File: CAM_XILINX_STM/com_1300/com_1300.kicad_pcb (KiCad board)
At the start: 6 copper layers, 50 x 75.9 mm, 113 parts, among them IC1 XC3S400-4TQ144C, J1 MEC1-108-01-S-D-RA1-SL, J2 Conn_02x10_Top_Bottom, J3 9-68RD-0.635SF, U1 LT1963AxST-3.3, U2 LP3982IMM-ADJ, U3 LTC3411EMS, U4 STM32F415RGTx, U5 AM29LV320DT90EC, U6 TC74LCX373FT, Y1 40mHZ, Y2 16mHz

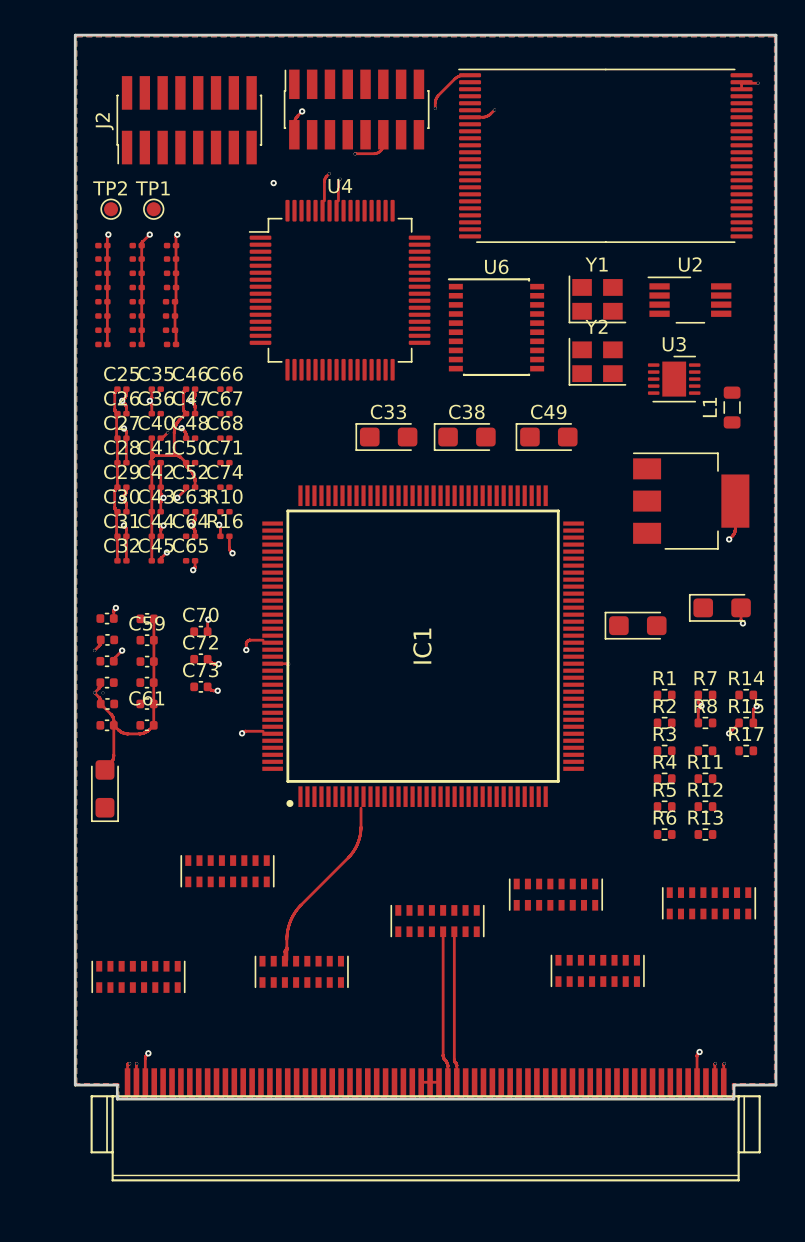
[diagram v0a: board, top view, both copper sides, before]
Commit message: 23623637
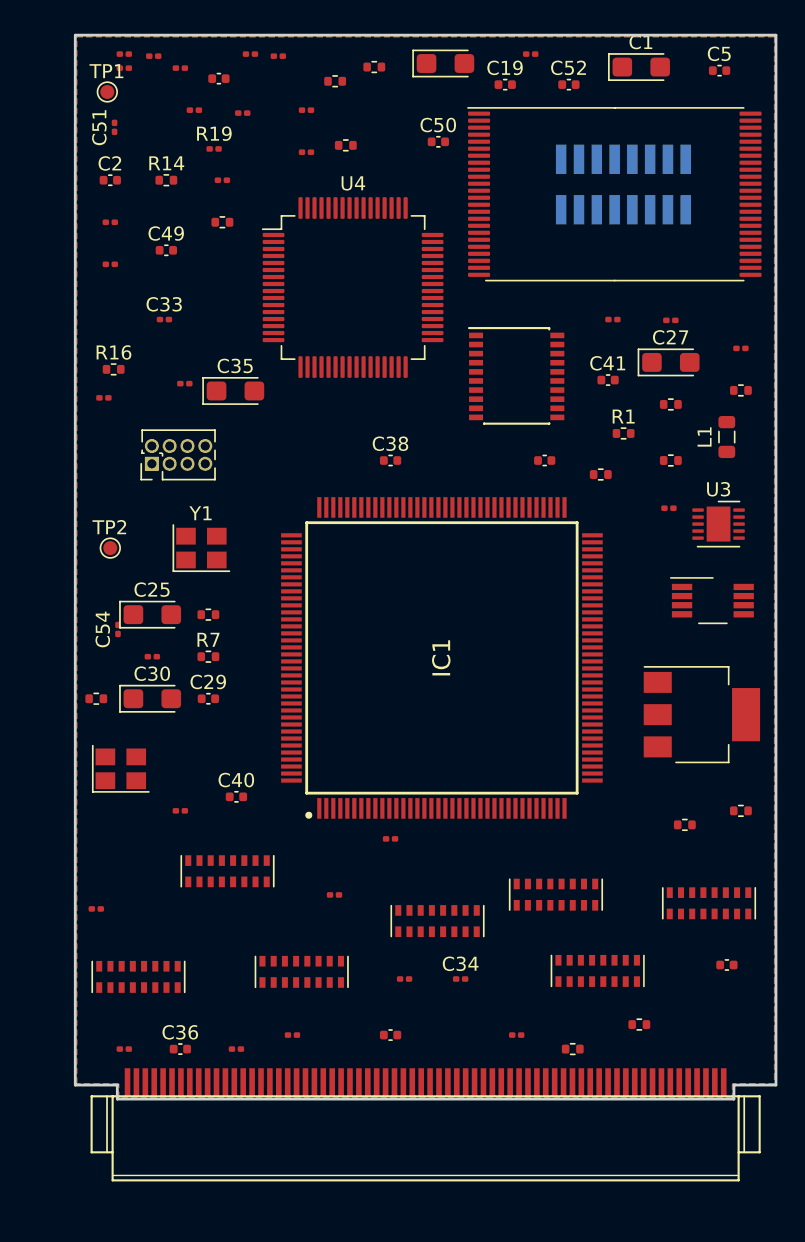
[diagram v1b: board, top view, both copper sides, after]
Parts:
- removed the C24 at (41.5, 66.2)
- removed the C24 at (40.7, 61.2)
- removed the C24 at (37.6, 71.4)
- removed the C24 at (43.2, 55.9)
- removed the C24 at (40.7, 57.7)
- removed the C24 at (37.6, 72.9)
- removed the C24 at (43.2, 54.2)
- removed the C24 at (43.2, 52.4)
- removed the C24 at (41.5, 68.2)
- removed the C24 at (40.7, 59.4)
- removed the C24 at (43.2, 50.7)
- removed the C24 at (43.2, 48.9)
- removed the C24 at (41.5, 70.2)
- removed C55: 10uF, Capacitor_Tantalum_SMD:CP_EIA-3216-18_Kemet-A
- removed C56: 4.7uF, Capacitor_SMD:C_0402_1005Metric
- removed C57, C58, C59, C60, C61: C-OPEN, Capacitor_SMD:C_0402_1005Metric
- added R18: 0, Resistor_SMD:R_0402_1005Metric, F.Cu at (51.0, 26.9)
- added R19: 0, Resistor_SMD:R_0201_0603Metric, F.Cu at (42.4, 31.8)
- added R20: 47, Resistor_SMD:R_0402_1005Metric, F.Cu at (51.8, 31.5)
- C1, C18, C25, C27, C30: renamed from C24; value C-OPEN -> 10uF; footprint Capacitor_SMD:C_0201_0603Metric -> Capacitor_Tantalum_SMD:CP_EIA-3216-18_Kemet-A
- C24: renamed from C50; value 22pF -> C-OPEN; footprint Capacitor_SMD:C_0201_0603Metric -> Capacitor_SMD:C_0402_1005Metric
- C24: renamed from C48; value 100nF -> C-OPEN
- C24 (x3): footprint Capacitor_SMD:C_0201_0603Metric -> Capacitor_SMD:C_0402_1005Metric
- C24: renamed from C49; value 10uF -> C-OPEN; footprint Capacitor_Tantalum_SMD:CP_EIA-3216-18_Kemet-A -> Capacitor_SMD:C_0402_1005Metric
- C24: footprint Capacitor_SMD:C_0402_1005Metric -> Capacitor_SMD:C_0201_0603Metric
- C24: renamed from C33; value 10uF -> C-OPEN; footprint Capacitor_Tantalum_SMD:CP_EIA-3216-18_Kemet-A -> Capacitor_SMD:C_0201_0603Metric
- C24: renamed from C51; value 10uF -> C-OPEN; footprint Capacitor_Tantalum_SMD:CP_EIA-3216-18_Kemet-A -> Capacitor_SMD:C_0201_0603Metric
- C24: renamed from C52; value 100nF -> C-OPEN; footprint Capacitor_SMD:C_0201_0603Metric -> Capacitor_SMD:C_0402_1005Metric
- C24: value C-OPEN -> 100nF
- C24: renamed from C53; value 4.7uF -> C-OPEN
- C24: renamed from C54; value 10uF -> C-OPEN; footprint Capacitor_Tantalum_SMD:CP_EIA-3216-18_Kemet-A -> Capacitor_SMD:C_0201_0603Metric
- C26: renamed from C24; value C-OPEN -> 22pF
- C28, C4: renamed from C24; value C-OPEN -> 100nF
- C29, C5: renamed from C24; value C-OPEN -> 4.7uF; footprint Capacitor_SMD:C_0201_0603Metric -> Capacitor_SMD:C_0402_1005Metric
- C3: renamed from C24; value C-OPEN -> 1nF
- C35: value 1nF -> 10uF; footprint Capacitor_SMD:C_0201_0603Metric -> Capacitor_Tantalum_SMD:CP_EIA-3216-18_Kemet-A
- C36: value 100nF -> 4.7uF; footprint Capacitor_SMD:C_0201_0603Metric -> Capacitor_SMD:C_0402_1005Metric
- C37: value 4.7uF -> C-OPEN
- C38: value 10uF -> C-OPEN; footprint Capacitor_Tantalum_SMD:CP_EIA-3216-18_Kemet-A -> Capacitor_SMD:C_0402_1005Metric
- C40, C41: renamed from C24; footprint Capacitor_SMD:C_0201_0603Metric -> Capacitor_SMD:C_0402_1005Metric
- J1: value MEC1-108-01-S-D-RA1-SL -> Conn_02x04_Top_Bottom; footprint Connector_PinSocket_1.27mm:PinSocket_2x08_P1.27mm_Vertical_SMD -> Connector_PinHeader_1.27mm:PinHeader_2x04_P1.27mm_Vertical
- J2: value Conn_02x10_Top_Bottom -> MEC1-108-01-S-D-RA1-SL; footprint Connector_PinHeader_1.27mm:PinHeader_2x08_P1.27mm_Vertical_SMD -> Connector_PinSocket_1.27mm:PinSocket_2x08_P1.27mm_Vertical_SMD; moved to B.Cu
- R14: value 10K -> 330
- R15: value 0 -> 56
- R17: value 47 -> 10K
- R22: renamed from R12; value 330 -> 56
- R22: renamed from R16; value 0 -> 56; footprint Resistor_SMD:R_0201_0603Metric -> Resistor_SMD:R_0402_1005Metric
- moved R14 55.3 mm to (39.0, 34.0)
- moved R22 54.2 mm to (53.8, 25.9)
- moved R11 52.6 mm to (43.0, 37.0)
- moved C24 51.1 mm to (56.0, 91.0)
- moved C24 50.5 mm to (48.0, 95.0)
- moved C28 49.6 mm to (64.0, 95.0)
- moved C39 49.3 mm to (79.0, 90.0)
- moved C24 47.2 mm to (35.3, 30.2)
- moved C5 47.0 mm to (78.5, 26.2)
- moved R17 46.5 mm to (34.0, 71.0)
- moved C24 45.6 mm to (36.0, 96.0)
- moved C36 45.4 mm to (40.0, 96.0)
- moved Y2 44.7 mm to (35.8, 76.0)
- moved C24 44.5 mm to (51.0, 85.0)
- moved C24 43.5 mm to (80.0, 46.0)
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- renumbered C24 to C39, R13 to R22
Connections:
- C1 pad 1: +3V3 -> VCC
- C18 pad 1: +3V3 -> VCC
- C24 pad 1: +2V5 -> +1V2 (x2)
- C24 pad 1: +1V2 -> +3V3 (x6)
- C24 pad 1: +1V2 -> Net-(U4-VCAP_2)
- C24 pad 2: Net-(U3-VFB) -> GND
- C24 pad 1: GND -> NRST
- C24 pad 2: Net-(U2-CC) -> GND
- C24 pad 1: +1V2 -> uC_CNTRL2
- C24 pad 1: +3V3 -> +2V5 (x4)
- C24 pad 1: +3V3 -> Net-(U4-VCAP_1)
- C24 pad 1: +3V3 -> Net-(C19-Pad1)
- C24 pad 1: +3V3 -> +1V2
- C24 pad 1: VCC -> +1V2
- C24 pad 1: GND -> OSC_IN
- C24 pad 2: +1V2 -> GND
- C24 pad 1: +3V3 -> GND
- C24 pad 2: GND -> Net-(U2-CC)
- C24 pad 1: GND -> Net-(C53-Pad1)
- C24 pad 2: +2V5 -> GND
- C25 pad 1: +2V5 -> +3V3
- C26 pad 1: +2V5 -> +1V2
- C26 pad 2: GND -> Net-(U3-VFB)
- C27 pad 1: +2V5 -> +3V3
- C28 pad 1: +2V5 -> GND
- C28 pad 2: GND -> +1V2
- C29 pad 1: +2V5 -> GND
- C29 pad 2: GND -> +2V5
- C3 pad 1: +3V3 -> GND
- C3 pad 2: GND -> Net-(C3-Pad2)
- C30 pad 1: +2V5 -> +1V2
- C35 pad 1: GND -> +1V2
- C35 pad 2: Net-(C35-Pad2) -> GND
- C36 pad 2: VCC -> +1V2
- C37 pad 1: GND -> /FPGA_CLK1
- C37 pad 2: VCC -> GND
- C38 pad 1: VCC -> GND
- C38 pad 2: GND -> uC_CNTRL1
- C39 pad 1: Net-(C39-Pad1) -> 40MHz_OSC
- C4 pad 1: +3V3 -> GND
- C4 pad 2: GND -> VCC
- C40 pad 1: +1V2 -> GND
- C40 pad 2: GND -> uC_CNTRL2
- C41 pad 1: +1V2 -> GND
- C41 pad 2: GND -> uC_CNTRL4
- C5 pad 1: +3V3 -> GND
- C5 pad 2: GND -> VCC
- J1 pad 2: GND -> Net-(J1-Pin_2)
- J1 pad 3: SERIAL_RX -> Net-(J1-Pin_3)
- J1 pad 4: SERIAL_TX -> Net-(IC1-TDO)
- J1 pad 5: unconnected-(J1-Pad5) -> GND
- J1 pad 6: unconnected-(J1-Pad6) -> Net-(J1-Pin_6)
- J1 pad 7: FPGA_TEST_EDGE1 -> unconnected-(J1-Pin_7-Pad7)
- J1 pad 8: FPGA_TEST_EDGE2 -> unconnected-(J1-Pin_8-Pad8)
- J2 pad 1: unconnected-(J2-Pin_1-Pad1) -> +3V3
- J2 pad 10: unconnected-(J2-Pin_10-Pad10) -> FPGA_TEST_EDGE4
- J2 pad 11: unconnected-(J2-Pin_11-Pad11) -> FPGA_TEST_EDGE5
- J2 pad 12: unconnected-(J2-Pin_12-Pad12) -> FPGA_TEST_EDGE6
- J2 pad 13: unconnected-(J2-Pin_13-Pad13) -> uC_PROG1
- J2 pad 14: unconnected-(J2-Pin_14-Pad14) -> NRST
- J2 pad 15: unconnected-(J2-Pin_15-Pad15) -> uC_PROG2
- J2 pad 16: unconnected-(J2-Pin_16-Pad16) -> uC_PROG4
- J2 pad 2: unconnected-(J2-Pin_2-Pad2) -> GND
- J2 pad 3: unconnected-(J2-Pin_3-Pad3) -> SERIAL_RX
- J2 pad 4: unconnected-(J2-Pin_4-Pad4) -> SERIAL_TX
- J2 pad 7: unconnected-(J2-Pin_7-Pad7) -> FPGA_TEST_EDGE1
- J2 pad 8: unconnected-(J2-Pin_8-Pad8) -> FPGA_TEST_EDGE2
- J2 pad 9: unconnected-(J2-Pin_9-Pad9) -> FPGA_TEST_EDGE3
- R1 pad 2: Net-(C35-Pad2) -> Net-(C3-Pad2)
- R14 pad 1: NRST -> +2V5
- R14 pad 2: +3V3 -> FPGA_CNTRL3
- R15 pad 1: Net-(J3-CD1#) -> uC_CNTRL2
- R15 pad 2: GND -> Net-(IC1-CCLK)
- R17 pad 1: OSC_OUT -> NRST
- R17 pad 2: Net-(C73-Pad1) -> +3V3
- R2 pad 2: Net-(C39-Pad1) -> Net-(C19-Pad1)
- R22 pad 1: uC_CNTRL2 -> Net-(J1-Pin_3)
- R22 pad 2: Net-(IC1-CCLK) -> Net-(IC1-TCK)
- R22 pad 1: +2V5 -> Net-(J1-Pin_2)
- R22 pad 2: FPGA_CNTRL3 -> Net-(IC1-TMS)
- R22 pad 1: GND -> TDI
- R22 pad 2: Net-(J3-CD2#) -> Net-(J1-Pin_6)
- Y1 pad 3: Net-(C39-Pad1) -> Net-(C19-Pad1)
- Y2 pad 3: Net-(C73-Pad1) -> Net-(C53-Pad1)
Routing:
- net GND: track 89.5 -> 0.00 mm, vias 38 -> 0
- net FPGA_TEST_EDGE6: track 42.5 -> 0.00 mm, vias 2 -> 0
- net Net-(J3-CD2#): track 41.6 -> 0.00 mm, vias 2 -> 0
- net Net-(J3-CD1#): track 26.8 -> 0.00 mm, vias 2 -> 0
- net +1V2: track 21.7 -> 0.00 mm
- net uC_A10: track 16.4 -> 0.00 mm, vias 2 -> 0
- net uC_A16: track 15.3 -> 0.00 mm, vias 2 -> 0
- net INOUT_A5: track 14.0 -> 0.00 mm
- net +2V5: track 12.5 -> 0.00 mm
- net MDI3: track 10.8 -> 0.00 mm
- net IREQ#: track 10.8 -> 0.00 mm
- net +3V3: track 1.78 -> 0.00 mm, vias 1 -> 0
- net VCC: track 1.27 -> 0.00 mm
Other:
- copper layers 6 -> 4

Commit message: 2234545
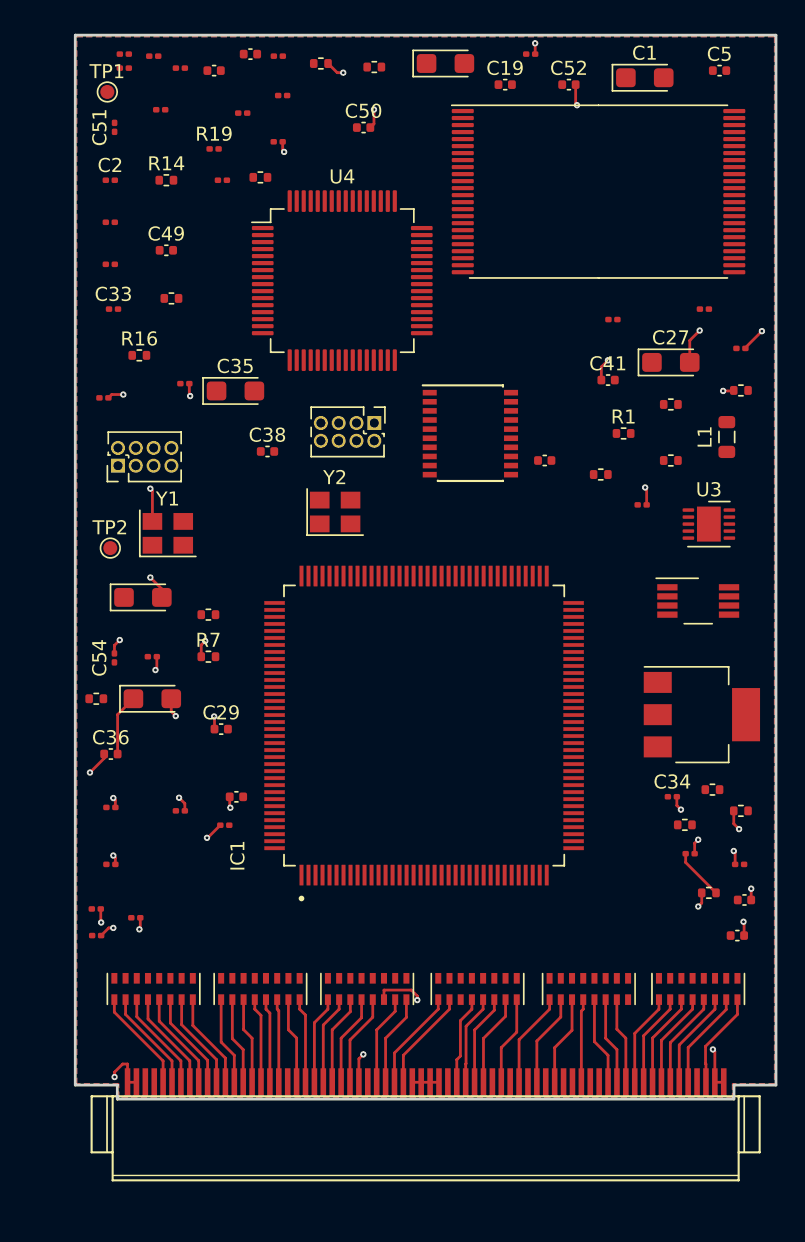
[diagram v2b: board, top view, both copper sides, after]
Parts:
- removed RN7: 8 x 180R, Resistor_SMD:R_Cat16-8
- C2: renamed from C24; value C-OPEN -> 1nF; footprint Capacitor_SMD:C_0402_1005Metric -> Capacitor_SMD:C_0201_0603Metric
- C24: renamed from C3; value 1nF -> C-OPEN; footprint Capacitor_SMD:C_0201_0603Metric -> Capacitor_SMD:C_0402_1005Metric
- IC1: footprint SUNfWGlsaW54X1hDM1MyMDAtNFRRRzE0NEMuemlw:QFP50P2200X2200X160-144N -> QFP50P2200X2200X160-144N:QFP50P2200X2200X160-144N
- J2: value MEC1-108-01-S-D-RA1-SL -> Conn_02x04_Top_Bottom; footprint Connector_PinSocket_1.27mm:PinSocket_2x08_P1.27mm_Vertical_SMD -> Connector_PinHeader_1.27mm:PinHeader_2x04_P1.27mm_Vertical; moved to F.Cu
- R2: value 47 -> 220K
- R3: value 220K -> 47
- moved RN5 34.6 mm to (77.0, 91.7)
- moved RN3 29.5 mm to (38.1, 91.7)
- moved C37 27.0 mm to (80.3, 85.4)
- moved J2 24.6 mm to (53.8, 51.3)
- moved Y2 23.9 mm to (51.0, 57.7)
- moved C24 22.3 mm to (76.4, 82.1)
- moved C36 21.6 mm to (35.0, 74.9)
- moved R15 21.0 mm to (78.0, 77.5)
- moved RN2 20.5 mm to (69.1, 91.7)
- moved C28 20.0 mm to (79.9, 82.8)
- moved C24 19.9 mm to (75.1, 78.0)
- moved RN4 17.6 mm to (61.2, 91.7)
- moved C24 17.3 mm to (35.0, 78.8)
- moved RN1 16.3 mm to (53.3, 91.7)
- moved C24 16.1 mm to (35.0, 82.8)
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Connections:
- C2 pad 1: +3V3 -> GND
- C2 pad 2: GND -> Net-(C2-Pad2)
- C24 pad 1: GND -> +3V3
- C24 pad 2: Net-(C3-Pad2) -> GND
- IC1 pad 10: INOUT_A5 -> INOUT_A4
- IC1 pad 105: INOUT_RESET -> INOUT_MCLKI
- IC1 pad 107: INOUT_WE# -> unconnected-(IC1-IO_L01P_2/VRN_2-Pad107)
- IC1 pad 108: INOUT_MCLKI -> unconnected-(IC1-IO_L01N_2/VRP_2-Pad108)
- IC1 pad 109: unconnected-(IC1-TDO-Pad109) -> Net-(IC1-TDO)
- IC1 pad 11: INOUT_A4 -> INOUT_A3
- IC1 pad 110: unconnected-(IC1-TCK-Pad110) -> Net-(IC1-TCK)
- IC1 pad 111: unconnected-(IC1-TMS-Pad111) -> Net-(IC1-TMS)
- IC1 pad 12: INOUT_A3 -> INOUT_A2
- IC1 pad 129: FPGA_TEST_EDGE6 -> unconnected-(IC1-IO_L31P_0/VREF_0-Pad129)
- IC1 pad 13: INOUT_A2 -> INOUT_A1
- IC1 pad 130: FPGA_TEST_EDGE5 -> INOUT_MISTRT
- IC1 pad 131: FPGA_TEST_EDGE4 -> INOUT_IOWR#
- IC1 pad 132: FPGA_TEST_EDGE3 -> INOUT_IORD#
- IC1 pad 135: FPGA_TEST_EDGE2 -> INOUT_RESET
- IC1 pad 137: FPGA_TEST_EDGE1 -> INOUT_WE#
- IC1 pad 14: INOUT_A1 -> INOUT_A0
- IC1 pad 144: unconnected-(IC1-TDI-Pad144) -> TDI
- IC1 pad 15: INOUT_A0 -> INOUT_INPACK#
- IC1 pad 17: unconnected-(IC1-IO_L40P_7-Pad17) -> INOUT_REG#
- IC1 pad 20: INOUT_INPACK# -> unconnected-(IC1-IO_L40P_6/VREF_6-Pad20)
- IC1 pad 21: INOUT_REG# -> INOUT_MOVAL
- IC1 pad 23: INOUT_MOVAL -> INOUT_MIVAL
- IC1 pad 24: INOUT_MIVAL -> INOUT_MDO7
- IC1 pad 25: INOUT_MDO7 -> INOUT_MDO6
- IC1 pad 26: INOUT_MDO6 -> INOUT_MDO5
- IC1 pad 27: INOUT_MDO5 -> INOUT_MDO4
- IC1 pad 28: INOUT_MDO4 -> INOUT_MDO3
- IC1 pad 30: INOUT_MDO3 -> INOUT_MDO2
- IC1 pad 31: INOUT_MDO2 -> INOUT_MDO1
- IC1 pad 32: INOUT_MDO1 -> INOUT_MDO0
- IC1 pad 33: INOUT_MDO0 -> INOUT_IREQ#
- IC1 pad 5: unconnected-(IC1-IO_L20P_7-Pad5) -> INOUT_MCLKO
- IC1 pad 53: INOUT_MCLKI -> unconnected-(IC1-IO_L32N_5/GCLK3-Pad53)
- IC1 pad 6: INOUT_MCLKO -> INOUT_A7
- IC1 pad 7: INOUT_A7 -> INOUT_A6
- IC1 pad 77: INOUT_IREQ# -> INOUT_D0
- IC1 pad 78: INOUT_D0 -> INOUT_D1
- IC1 pad 79: INOUT_D1 -> INOUT_D2
- IC1 pad 8: INOUT_A6 -> INOUT_A5
- IC1 pad 80: INOUT_D2 -> INOUT_D3
- IC1 pad 82: INOUT_D3 -> INOUT_D4
- IC1 pad 83: INOUT_D4 -> INOUT_D5
- IC1 pad 84: INOUT_D5 -> unconnected-(IC1-IO_L23P_3/VREF_3-Pad84)
- IC1 pad 90: INOUT_CE1# -> unconnected-(IC1-IO_L40N_3/VREF_3-Pad90)
- IC1 pad 92: INOUT_MISTRT -> unconnected-(IC1-IO_L40P_2/VREF_2-Pad92)
- IC1 pad 93: INOUT_IOWR# -> INOUT_CE1#
- IC1 pad 95: INOUT_IORD# -> INOUT_MDI0
- IC1 pad 96: INOUT_MDI0 -> INOUT_MDI1
- IC1 pad 97: INOUT_MDI1 -> INOUT_MDI2
- IC1 pad 98: INOUT_MDI2 -> unconnected-(IC1-IO_L23N_2/VREF_2-Pad98)
- J1 pad 1: +3V3 -> Net-(J1-Pin_1)
- J1 pad 6: Net-(J1-Pin_6) -> GND
- J1 pad 7: unconnected-(J1-Pin_7-Pad7) -> GND
- J1 pad 8: unconnected-(J1-Pin_8-Pad8) -> +3V3
- J2 pad 2: GND -> SERIAL_RX
- J2 pad 3: SERIAL_RX -> uC_PROG1
- J2 pad 4: SERIAL_TX -> uC_PROG2
- J2 pad 5: unconnected-(J2-Pad5) -> GND
- J2 pad 6: unconnected-(J2-Pad6) -> SERIAL_TX
- J2 pad 7: FPGA_TEST_EDGE1 -> NRST
- J2 pad 8: FPGA_TEST_EDGE2 -> uC_PROG4
- R1 pad 2: Net-(C3-Pad2) -> Net-(C2-Pad2)
- R2 pad 1: 40MHz_OSC -> GND
- R2 pad 2: Net-(C19-Pad1) -> Net-(U3-SHDN/RT)
- R22 pad 2: Net-(J1-Pin_6) -> Net-(J1-Pin_1)
- R3 pad 1: GND -> 40MHz_OSC
- R3 pad 2: Net-(U3-SHDN/RT) -> Net-(C19-Pad1)
- RN1 pad 1: INOUT_MOSTRT -> INOUT_MCLKI
- RN1 pad 10: MDO2 -> MCLKO
- RN1 pad 11: D2 -> A6
- RN1 pad 12: MDO1 -> MDI7
- RN1 pad 13: D1 -> A7
- RN1 pad 14: MDO0 -> MDI6
- RN1 pad 15: D0 -> MDI5
- RN1 pad 16: MOSTRT -> MCLKI
- RN1 pad 2: INOUT_D0 -> INOUT_MDI5
- RN1 pad 3: INOUT_MDO0 -> INOUT_MDI6
- RN1 pad 4: INOUT_D1 -> INOUT_A7
- RN1 pad 5: INOUT_MDO1 -> INOUT_MDI7
- RN1 pad 6: INOUT_D2 -> INOUT_A6
- RN1 pad 7: INOUT_MDO2 -> INOUT_MCLKO
- RN1 pad 8: unconnected-(RN1-R8.1-Pad8) -> INOUT_A5
- RN1 pad 9: unconnected-(RN1-R8.2-Pad9) -> A5
- RN2 pad 1: INOUT_MCLKO -> unconnected-(RN2-R1.1-Pad1)
- RN2 pad 10: RESET -> IOWR#
- RN2 pad 11: A5 -> IORD#
- RN2 pad 12: A6 -> OE#
- RN2 pad 13: MDI7 -> MDO7
- RN2 pad 14: A7 -> CE1#
- RN2 pad 15: MDI6 -> MDO6
- RN2 pad 16: MCLKO -> unconnected-(RN2-R1.2-Pad16)
- RN2 pad 2: INOUT_MDI6 -> INOUT_MDO6
- RN2 pad 3: INOUT_A7 -> INOUT_CE1#
- RN2 pad 4: INOUT_MDI7 -> INOUT_MDO7
- RN2 pad 5: INOUT_A6 -> INOUT_OE#
- RN2 pad 6: INOUT_A5 -> INOUT_IORD#
- RN2 pad 7: INOUT_RESET -> INOUT_IOWR#
- RN2 pad 8: INOUT_A4 -> INOUT_MISTRT
- RN2 pad 9: A4 -> MISTRT
- RN3 pad 1: unconnected-(RN3-R1.1-Pad1) -> INOUT_A0
- RN3 pad 10: unconnected-(RN3-R7.2-Pad10) -> D2
- RN3 pad 11: MDI0 -> MDO1
- RN3 pad 12: unconnected-(RN3-R5.2-Pad12) -> D1
- RN3 pad 13: MISTRT -> MDO0
- RN3 pad 14: unconnected-(RN3-R3.2-Pad14) -> D0
- RN3 pad 15: IOWR# -> MOSTRT
- RN3 pad 16: unconnected-(RN3-R1.2-Pad16) -> A0
- RN3 pad 2: INOUT_IOWR# -> INOUT_MOSTRT
- RN3 pad 3: unconnected-(RN3-R3.1-Pad3) -> INOUT_D0
- RN3 pad 4: INOUT_MISTRT -> INOUT_MDO0
- RN3 pad 5: unconnected-(RN3-R5.1-Pad5) -> INOUT_D1
- RN3 pad 6: INOUT_MDI0 -> INOUT_MDO1
- RN3 pad 7: unconnected-(RN3-R7.1-Pad7) -> INOUT_D2
- RN3 pad 8: INOUT_MDI1 -> INOUT_MDO2
- RN3 pad 9: MDI1 -> MDO2
- RN4 pad 1: INOUT_D3 -> INOUT_MDI0
- RN4 pad 10: MDO5 -> MIVAL
- RN4 pad 11: D6 -> MDI3
- RN4 pad 12: MDO4 -> IREQ#
- RN4 pad 13: D5 -> MDI2
- RN4 pad 14: MDO3 -> WE#
- RN4 pad 15: D4 -> MDI1
- RN4 pad 16: D3 -> MDI0
- RN4 pad 2: INOUT_D4 -> INOUT_MDI1
- RN4 pad 3: INOUT_MDO3 -> INOUT_WE#
- RN4 pad 4: INOUT_D5 -> INOUT_MDI2
- RN4 pad 5: INOUT_MDO4 -> INOUT_IREQ#
- RN4 pad 6: INOUT_D6 -> INOUT_MDI3
- RN4 pad 7: INOUT_MDO5 -> INOUT_MIVAL
- RN4 pad 8: INOUT_D7 -> INOUT_MDI4
- RN4 pad 9: D7 -> MDI4
- RN5 pad 1: unconnected-(RN5-R1.1-Pad1) -> INOUT_D3
- RN5 pad 10: MOVAL -> MDO5
- RN5 pad 11: A1 -> D6
- RN5 pad 12: REG# -> MDO4
- RN5 pad 13: A2 -> D5
- RN5 pad 14: INPACK# -> MDO3
- RN5 pad 15: A3 -> D4
- RN5 pad 16: unconnected-(RN5-R1.2-Pad16) -> D3
- RN5 pad 2: INOUT_A3 -> INOUT_D4
- RN5 pad 3: INOUT_INPACK# -> INOUT_MDO3
- RN5 pad 4: INOUT_A2 -> INOUT_D5
- RN5 pad 5: INOUT_REG# -> INOUT_MDO4
- RN5 pad 6: INOUT_A1 -> INOUT_D6
- RN5 pad 7: INOUT_MOVAL -> INOUT_MDO5
- RN5 pad 8: INOUT_A0 -> INOUT_D7
- RN5 pad 9: A0 -> D7
- RN6 pad 1: INOUT_WE# -> INOUT_RESET
- RN6 pad 10: MCLKI -> A1
- RN6 pad 11: MDI4 -> REG#
- RN6 pad 12: MIVAL -> A2
- RN6 pad 13: MDI3 -> INPACK#
- RN6 pad 14: IREQ# -> A3
- RN6 pad 15: MDI2 -> A4
- RN6 pad 16: WE# -> RESET
- RN6 pad 2: INOUT_MDI2 -> INOUT_A4
- RN6 pad 3: INOUT_IREQ# -> INOUT_A3
- RN6 pad 4: INOUT_MDI3 -> INOUT_INPACK#
- RN6 pad 5: INOUT_MIVAL -> INOUT_A2
- RN6 pad 6: INOUT_MDI4 -> INOUT_REG#
- RN6 pad 7: INOUT_MCLKI -> INOUT_A1
- RN6 pad 8: INOUT_MDI5 -> INOUT_MOVAL
- RN6 pad 9: MDI5 -> MOVAL
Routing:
- net GND: track 0.00 -> 48.9 mm, vias 0 -> 37
- net MDI6: track 0.00 -> 11.1 mm, vias 0 -> 2
- net MDO2: track 0.00 -> 7.34 mm
- net D2: track 0.00 -> 7.27 mm
- net MIVAL: track 0.00 -> 7.26 mm
- net MDO1: track 0.00 -> 7.20 mm
- net MDI4: track 0.00 -> 7.19 mm
- net D1: track 0.00 -> 7.13 mm
- net MDO0: track 0.00 -> 7.07 mm
- net D4: track 0.00 -> 7.02 mm
- net D0: track 0.00 -> 7.00 mm
- net MDO3: track 0.00 -> 6.96 mm
- net MOSTRT: track 0.00 -> 6.93 mm
- net D5: track 0.00 -> 6.89 mm
- net A0: track 0.00 -> 6.86 mm
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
